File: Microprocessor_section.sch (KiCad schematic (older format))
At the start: 14 parts, among them J15 Conn_01x06_Male, SW1 K2-1102SP-C4SC-04, U5 ESP32-WROOM-32D

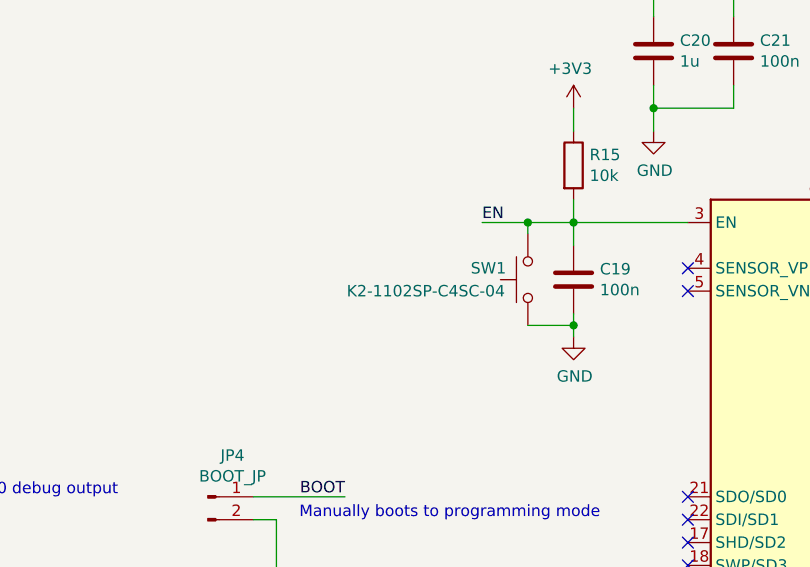
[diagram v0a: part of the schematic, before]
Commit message: Start PCB layout
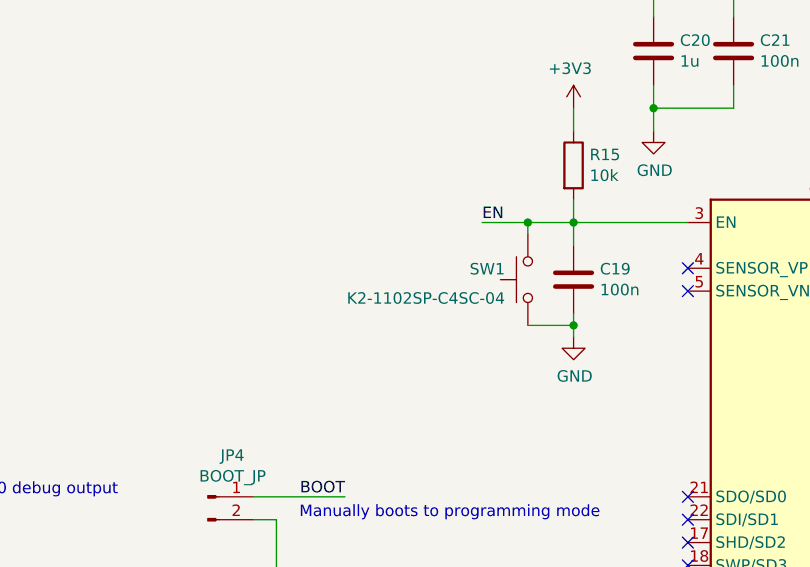
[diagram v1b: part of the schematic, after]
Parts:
- removed SW1: K2-1102SP-C4SC-04, co2_sensor_node:K2-1102SP-xxxC, symbol Switch:SW_MEC_5G
- added SW1: K2-1102SP-C4SC-04, co2_sensor_node:K2-1102SP-xxxC, symbol Switch:SW_Push
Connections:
- net EN: now also SW1.2
- net GND: now also SW1.1
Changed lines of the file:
@@
 Text HLabel 7600 3500 2    50   Output ~ 0
 UART1_TX
-$Comp
-L Switch:SW_MEC_5G SW1
-U 1 1 60A91701
-P 5200 3050
-F 0 "SW1" V 5150 3300 50  0000 R CNN
-F 1 "K2-1102SP-C4SC-04" V 5250 3150 50  0000 L CNN
-F 2 "co2_sensor_node:K2-1102SP-xxxC" H 5200 3250 50  0001 C CNN
-F 3 "https://datasheet.lcsc.com/szlcsc/1811082113_Korean-Hroparts-Elec-K2-1102SP-C4SC-04_C127509.pdf" H 5200 3250 50  0001 C CNN
-F 4 "https://lcsc.com/product-detail/Tactile-Switches_Korean-Hroparts-Elec-K2-1102SP-C4SC-04_C127509.html/?href=jlc-SMT" V 5200 3050 50  0001 C CNN "LCSC"
-	1    5200 3050
-	0    -1   1    0
-$EndComp
 Wire Wire Line
 	5200 2800 5200 2850
@@
 Wire Wire Line
 	2300 4100 2600 4100
+$Comp
+L Switch:SW_Push SW1
+U 1 1 60B19388
+P 5200 3050
+F 0 "SW1" V 5246 3150 50  0000 L CNN
+F 1 "K2-1102SP-C4SC-04" V 5118 3150 50  0000 L CNN
+F 2 "co2_sensor_node:K2-1102SP-xxxC" H 5200 3250 50  0001 C CNN
+F 3 "https://datasheet.lcsc.com/szlcsc/1811082113_Korean-Hroparts-Elec-K2-1102SP-C4SC-04_C127509.pdf" H 5200 3250 50  0001 C CNN
+F 4 "https://lcsc.com/product-detail/Tactile-Switches_Korean-Hroparts-Elec-K2-1102SP-C4SC-04_C127509.html/?href=jlc-SMT" V 5200 3050 50  0001 C CNN "LCSC"
+	1    5200 3050
+	0    -1   -1   0
+$EndComp
 $EndSCHEMATC
